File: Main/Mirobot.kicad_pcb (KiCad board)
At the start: 2 copper layers, 110 x 31.2 mm, 24 parts, among them IC1 ARDUINO_PRO_MINI, M1 ESP8266-ESP-12, P1 CONN_01X02, P3 RIGHT_STEPPER, P4 LEFT_STEPPER, SW1 POWER_SWITCH, SW2 LEFT_BUMP, SW3 RIGHT_BUMP, U2 ULN2803A

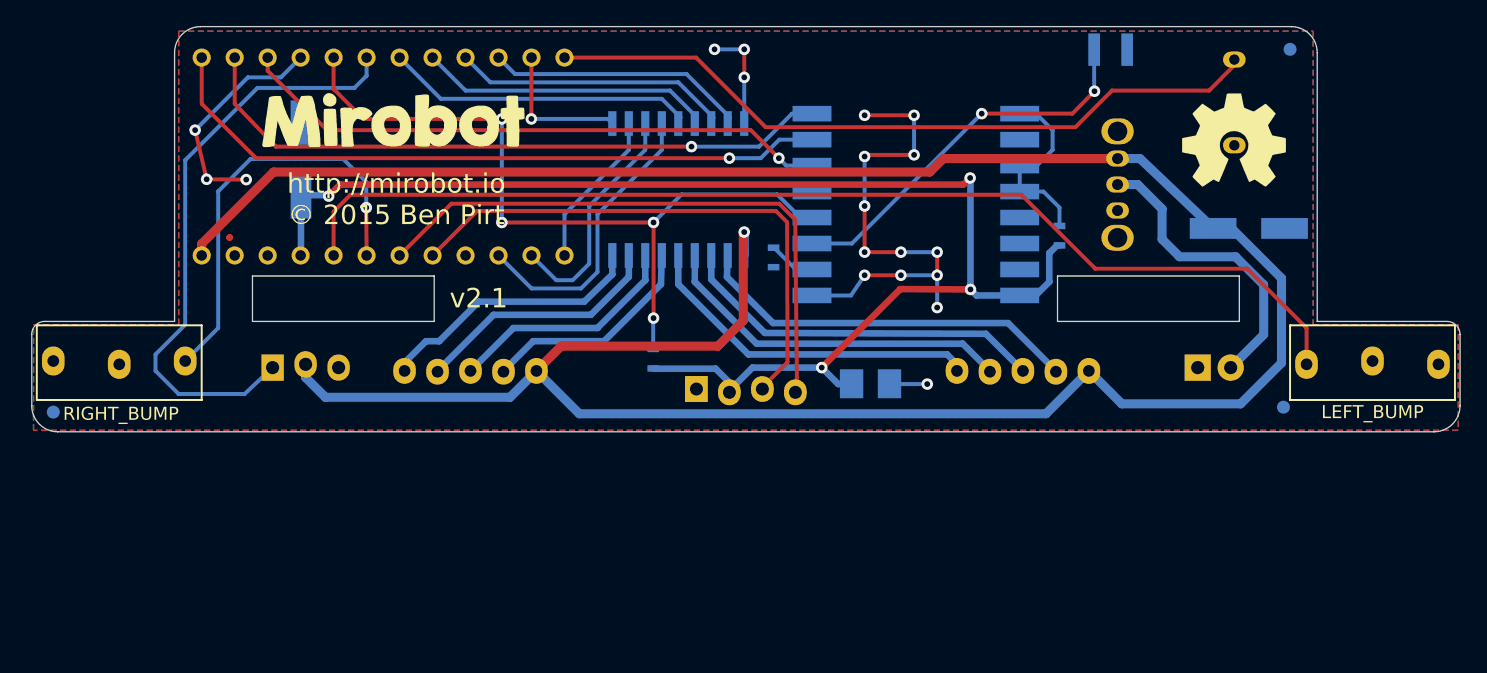
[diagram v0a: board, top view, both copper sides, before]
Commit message: initial version of v3.0
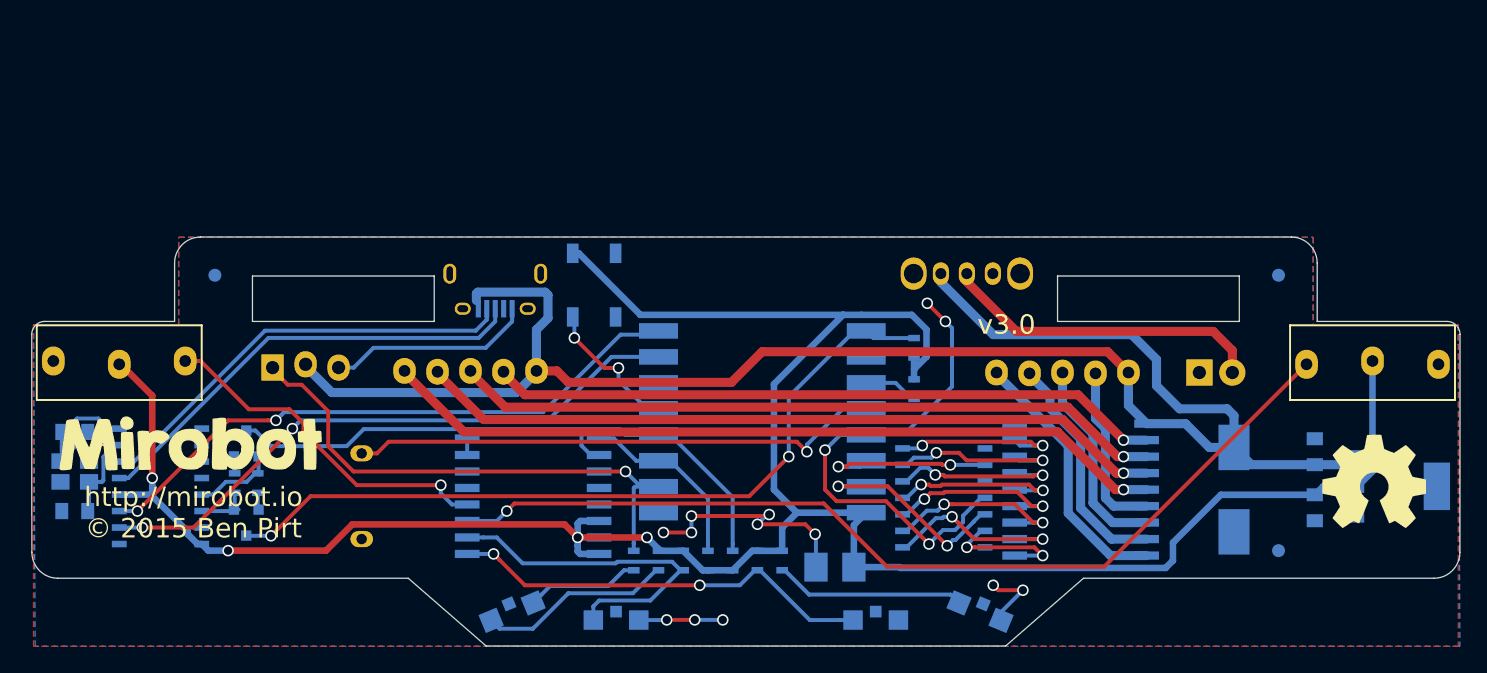
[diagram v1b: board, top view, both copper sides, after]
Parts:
- removed IC1: ARDUINO_PRO_MINI, Mirobot:ARDUINO_PRO_MINI
- removed LINE1: LINE, Mirobot:Pin_Header_Staggered_1x04
- removed P1: CONN_01X02, Mirobot:2-PIN-EDGE-CONN
- removed P4: LEFT_STEPPER, Mirobot:JST_XH-1x05
- added C6: 10uF, Capacitors_SMD:C_0805, B.Cu at (212.7, 137.0)
- added C7: 100uF, Capacitors_Tantalum_SMD:TantalC_SizeB_EIA-3528_Reflow, B.Cu at (175.8, 145.9)
- added C8: 10uF, Capacitors_SMD:C_0805, B.Cu at (212.7, 141.4)
- added D1: LED, Mirobot:SIDE-LED-REVERSED, B.Cu at (150.9, 149.4)
- added D2: LED, Mirobot:SIDE-LED-REVERSED, B.Cu at (186.9, 149.4)
- added L1: WS2812B, Mirobot:WS2812B, B.Cu at (157.2, 124.2)
- added P2: RIGHT_STEPPER, Mirobot:JST_XH-1x05, B.Cu at (193.3, 130.9)
- added Q1: S8050, TO_SOT_Packages_SMD:SOT-23, B.Cu at (130.4, 136.4)
- added Q2: S8050, TO_SOT_Packages_SMD:SOT-23, B.Cu at (130.4, 142.5)
- added R10: 10k, Resistors_SMD:R_0603, B.Cu at (129.5, 139.4)
- added R11: 10k, Resistors_SMD:R_0603, B.Cu at (131.3, 139.4)
- added R4: 10k, Resistors_SMD:R_0603, B.Cu at (167.9, 145.4)
- added R5: 10k, Resistors_SMD:R_0603, B.Cu at (166.0, 145.4)
- added R6: 20k, Resistors_SMD:R_0603, B.Cu at (169.8, 145.4)
- added R7: 160R, Resistors_SMD:R_0603, B.Cu at (162.2, 145.4)
- added R8: 20k, Resistors_SMD:R_0603, B.Cu at (164.1, 145.4)
- added R9: 160R, Resistors_SMD:R_0603, B.Cu at (171.7, 145.4)
- added U1: phototransistor, Mirobot:SIDE-LED, B.Cu at (178.9, 150.0)
- added U3: PCF8591, SMD_Packages:SO-16-L, B.Cu at (152.5, 140.5)
- added U4: 74HC595, SMD_Packages:SO-16-N, B.Cu at (184.2, 140.0)
- added U5: ULN2803A, Mirobot:SO-18, B.Cu at (194.7, 140.6)
- added U6: USB-A-PLUG, Connect:USB_Micro-B, B.Cu at (149.6, 124.5)
- added U7: CH340G, SMD_Packages:SO-16-N, B.Cu at (123.8, 139.7)
- added U8: LD1117S33CTR, TO_SOT_Packages_SMD:SOT-223, B.Cu at (218.8, 139.7)
- added X1: 12MHz, Crystals:crystal_FA238-TSX3225, B.Cu at (117.2, 138.6)
- C1, C2: value 470uF -> 22pF; footprint Capacitors_SMD:c_elec_6.3x7.7 -> Capacitors_SMD:C_0805
- C3: value 100uF -> 470uF; footprint Capacitors_Tantalum_SMD:TantalC_SizeB_EIA-3528_Reflow -> Capacitors_SMD:c_elec_8x10
- P3: value RIGHT_STEPPER -> LEFT_STEPPER
- SW1: value POWER_SWITCH -> LEFT_BUMP; footprint Mirobot:SMALL_SLIDE_SWITCH -> Mirobot:LEVER_SWITCH; moved to F.Cu
- SW2: value LEFT_BUMP -> RIGHT_BUMP
- SW3: value RIGHT_BUMP -> POWER_SWITCH; footprint Mirobot:LEVER_SWITCH -> Mirobot:SMALL_SLIDE_SWITCH; moved to B.Cu
- U2: value ULN2803A -> phototransistor; footprint Mirobot:SO-18 -> Mirobot:SIDE-LED
- moved C1 93.0 mm to (117.2, 141.6)
- moved SW1 78.1 mm to (120.7, 130.2), turned to 180 degrees
- moved SG1 73.7 mm to (139.3, 140.5)
- moved SW3 65.6 mm to (185.9, 123.3)
- moved FID3 38.6 mm to (209.9, 144.7)
- moved U2 33.4 mm to (158.9, 150.0), turned to 270 degrees
- moved ART1 29.4 mm to (126.1, 136.4)
- moved C3 29.2 mm to (206.5, 140.0), turned to 90 degrees
- moved ART2 28.4 mm to (217.3, 139.3)
- moved C2 27.3 mm to (117.2, 135.5), turned to 0 degrees
- moved R3 25.7 mm to (160.3, 145.4)
- moved M1 20.5 mm to (170.2, 133.7)
- moved R2 20.1 mm to (181.9, 129.0), turned to 270 degrees
- moved FID1 16.3 mm to (128.0, 123.4)
- moved R1 16.3 mm to (181.9, 132.2), turned to 90 degrees
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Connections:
- C1 pad 1: VSS -> Net-(C1-Pad1)
- C2 pad 1: +3V3 -> Net-(C2-Pad1)
- C3 pad 1: +3V3 -> VSS
- M1 pad 1: Net-(M1-Pad1) -> RESET
- M1 pad 10: Net-(M1-Pad10) -> SERVO
- M1 pad 11: Net-(M1-Pad11) -> SDA
- M1 pad 12: Net-(IC1-Pad5) -> SCL
- M1 pad 13: (no net) -> LED
- M1 pad 14: Net-(IC1-Pad3) -> GPIO5
- M1 pad 15: Net-(IC1-Pad1) -> RXD
- M1 pad 16: Net-(IC1-Pad2) -> TXD
- M1 pad 2: (no net) -> ADC
- M1 pad 3: Net-(M1-Pad1) -> CH_PD
- M1 pad 4: Net-(M1-Pad1) -> BUZZER
- M1 pad 5: (no net) -> SR_LATCH
- M1 pad 6: (no net) -> SR_DATA
- M1 pad 7: (no net) -> SR_CLK
- PEN1 pad 1: Net-(IC1-Pad6) -> SERVO
- R1 pad 1: Net-(M1-Pad1) -> CH_PD
- R2 pad 1: +3V3 -> RESET
- R2 pad 2: Net-(IC1-Pad5) -> +3V3
- R3 pad 2: Net-(M1-Pad10) -> SERVO
- SG1 pad 1: Net-(IC1-Pad12) -> BUZZER
- SW1 pad 1: VSS -> +3V3
- SW1 pad 2: Net-(BATT1-Pad2) -> Net-(SW1-Pad2)
- SW1 pad 3: (no net) -> GND
- SW2 pad 1: GND -> +3V3
- SW2 pad 3: (no net) -> GND
- SW3 pad 1: GND -> VSS
- SW3 pad 2: Net-(IC1-Pad19) -> Net-(BATT1-Pad2)
- SW3 pad 3: (no net) -> Net-(SW3-Pad3)
- U2 pad 2: Net-(IC1-Pad13) -> GND
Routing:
- net +3V3: track 107.6 -> 191.6 mm
- net VSS: track 206.0 -> 132.6 mm, vias 1 -> 0
- net RESET: track 0.00 -> 60.9 mm, vias 0 -> 2
- net Net-(IC1-Pad5): track 60.9 -> 0.00 mm, vias 4 -> 0
- net Net-(IC1-Pad12): track 56.2 -> 0.00 mm
- net Net-(IC1-Pad1): track 53.1 -> 0.00 mm, vias 1 -> 0
- net Net-(IC1-Pad2): track 50.5 -> 0.00 mm, vias 1 -> 0
- net RXD: track 0.00 -> 47.9 mm, vias 0 -> 2
- net SCL: track 0.00 -> 47.8 mm
- net TXD: track 0.00 -> 47.3 mm, vias 0 -> 2
- net Net-(IC1-Pad3): track 46.0 -> 0.00 mm, vias 1 -> 0
- net Net-(IC1-Pad18): track 45.8 -> 0.00 mm
- net Net-(IC1-Pad6): track 45.8 -> 0.00 mm
- net Net-(IC1-Pad17): track 43.3 -> 0.00 mm
- net SERVO: track 0.00 -> 42.0 mm, vias 0 -> 1
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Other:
- board size 110 x 31.2 mm -> 110 x 31.5 mm
- board text added: "v3.0"
- board text removed: "GND"
- board text removed: "LINE"
- board text removed: "The module above is based on the Pro Mini by Sparkfun"
- board text removed: "v2.1"
